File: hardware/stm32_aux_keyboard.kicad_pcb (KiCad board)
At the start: 2 copper layers, 95 x 95 mm, 156 parts, among them J1 I2C_HEADER,2.54, J3 BUZZER_HEADER, J4 ROT_ENC_HEADER, J5 SWD_SWD, J6 SWD_SWD, J7 ROT_ENC_HEADER, J8 I2C_HEADER,2.54, Q1 SS9013_J3, SW1 USR_BTN_1, SW10 KEY22, SW11 KEY23, SW12 KEY31, SW13 KEY32, SW14 KEY33, SW18 ROT1, SW19 SW_RESET,2_leg,SMD, SW2 USR_BTN_2, SW3 USR_BTN_3, SW4 USR_BTN_4, SW5 ROT2, SW6 KEY11, SW7 KEY12, SW8 KEY13, SW9 KEY21, U1 SSD1306-OLED-I2C, U10 STM32F103C8T6, U2 footprint-lib:AMS1117_SOT-223, U4 USB, U5 USBLC6-2SC6_SOT23-6, U6 STM32F103C8T6_rect, U7 SWD, U8 AMS1117-3.3, U9 USBLC6-2SC6_SOT23-6, Y1 O_8M, Y2 O8M, Y3 O32.768K

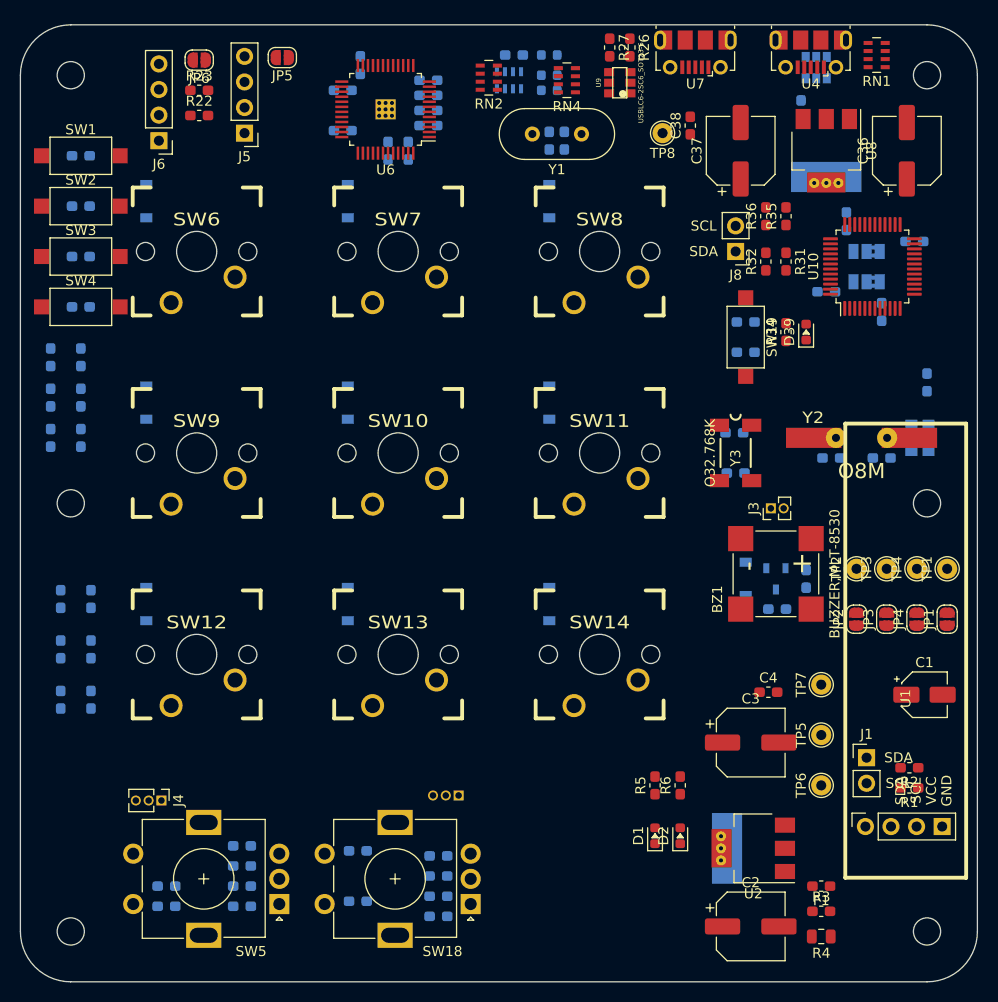
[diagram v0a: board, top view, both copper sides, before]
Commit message: update for routing,
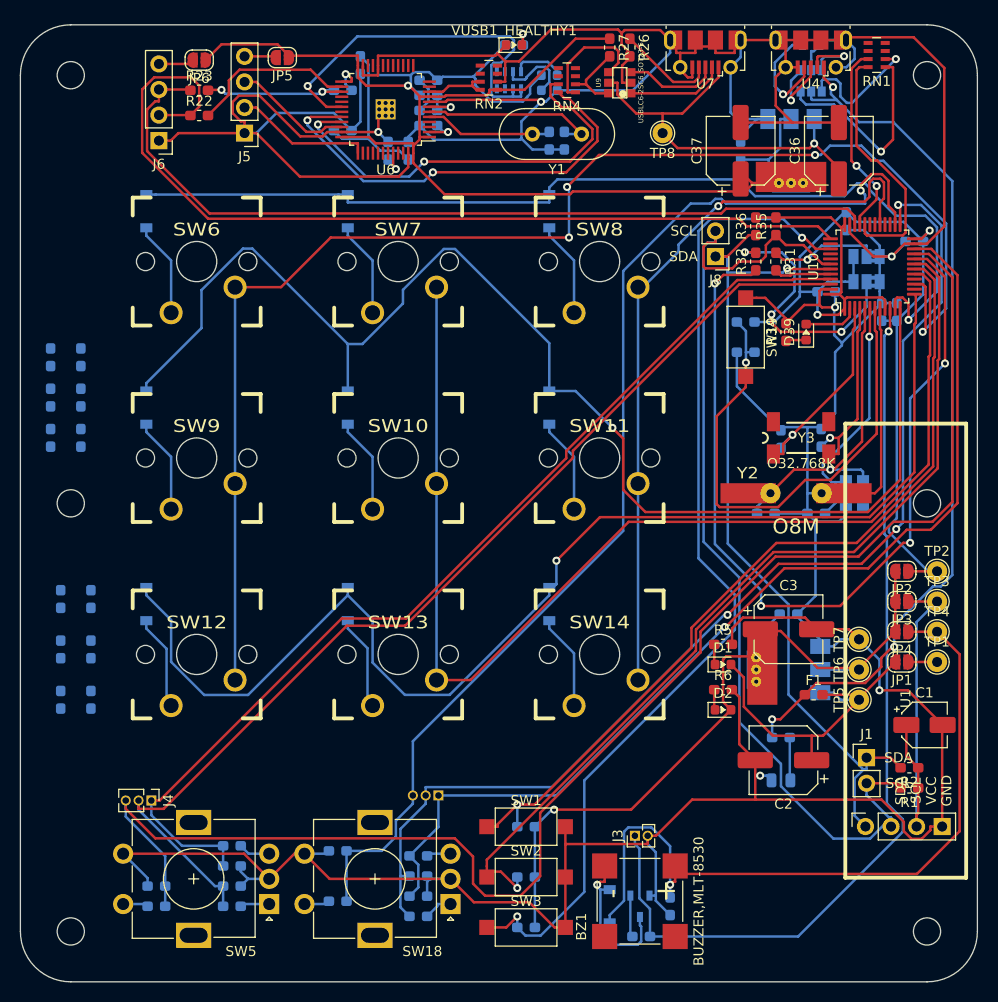
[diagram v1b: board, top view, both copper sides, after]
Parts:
- removed R13: R103,0603, Resistor_SMD:R_0603_1608Metric_Pad1.05x0.95mm_HandSolder
- removed SW4: USR_BTN_4, footprint-lib:SW_SPST_CK_RS282G05A3
- C38, C4, R3, R4, U8: moved to B.Cu
- U2: value footprint-lib:AMS1117_SOT-223 -> AMS1117-3.3; moved to B.Cu
- VUSB1_HEALTHY1: moved to F.Cu
- moved R10 79.9 mm to (70.2, 99.6)
- moved R11 79.9 mm to (70.2, 104.6)
- moved R12 79.9 mm to (70.2, 109.6)
- moved SW1 79.9 mm to (70.2, 99.6)
- moved SW2 79.9 mm to (70.2, 104.6)
- moved SW3 79.9 mm to (70.2, 109.6)
- moved R15 35.2 mm to (81.6, 110.5)
- moved BZ1 35.2 mm to (81.5, 107.0)
- moved D24 35.2 mm to (78.5, 107.5)
- moved J3 35.2 mm to (81.0, 100.5)
- moved Q1 35.2 mm to (81.5, 107.5)
- moved C25 35.2 mm to (84.5, 107.5)
- moved F1 19.0 mm to (98.8, 86.5), turned to 0 degrees
- moved D1 18.3 mm to (89.8, 83.5), turned to 0 degrees
- moved U2 18.1 mm to (96.2, 84.0)
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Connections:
- net Vws2812 renamed VCC
- C42 pad 1: +3V3 -> Vstm32
- J1 pad SCL: /SCL -> /oled/SCL
- J1 pad SDA: /SDA -> /oled/SDA
- R1 pad 2: /SCL -> /oled/SCL
- R2 pad 2: /SDA -> /oled/SDA
- U1 pad SCL: /SCL -> /oled/SCL
- U1 pad SDA: /SDA -> /oled/SDA
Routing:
- net GND: track 0.00 -> 589.7 mm, vias 0 -> 6
- net Vstm32_stlink: track 0.00 -> 161.5 mm, vias 0 -> 1
- net /stm32_core/ROT_ENC_SW1: track 0.00 -> 148.3 mm
- net /keyboard_key/COL1: track 0.00 -> 139.3 mm, vias 0 -> 4
- net /keyboard_key/ROW2: track 0.00 -> 131.5 mm, vias 0 -> 1
- net /keyboard_key/ROW3: track 0.00 -> 123.9 mm, vias 0 -> 1
- net /keyboard_key/COL2: track 0.00 -> 116.8 mm
- net /stm32_core/ROT_ENC_SW2: track 0.00 -> 113.3 mm, vias 0 -> 1
- net /rot_enc/B: track 0.00 -> 111.6 mm, vias 0 -> 3
- net Vstm32: track 0.00 -> 106.0 mm, vias 0 -> 2
- net /rot_enc2/B: track 0.00 -> 106.0 mm
- net /rot_enc/A: track 0.00 -> 103.5 mm, vias 0 -> 1
- net /oled/SCL: track 0.00 -> 102.5 mm
- net /stm32_core/USR_BTN3: track 0.00 -> 101.5 mm, vias 0 -> 2
- net /rot_enc2/A: track 0.00 -> 101.1 mm
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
